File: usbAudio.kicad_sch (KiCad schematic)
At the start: 35 parts, among them J1 USB_B_Micro, J2 54-00176, U1 PCM2906CDBR, U2 MAX9814, U3 TCR2EF36, Y1 12MHz

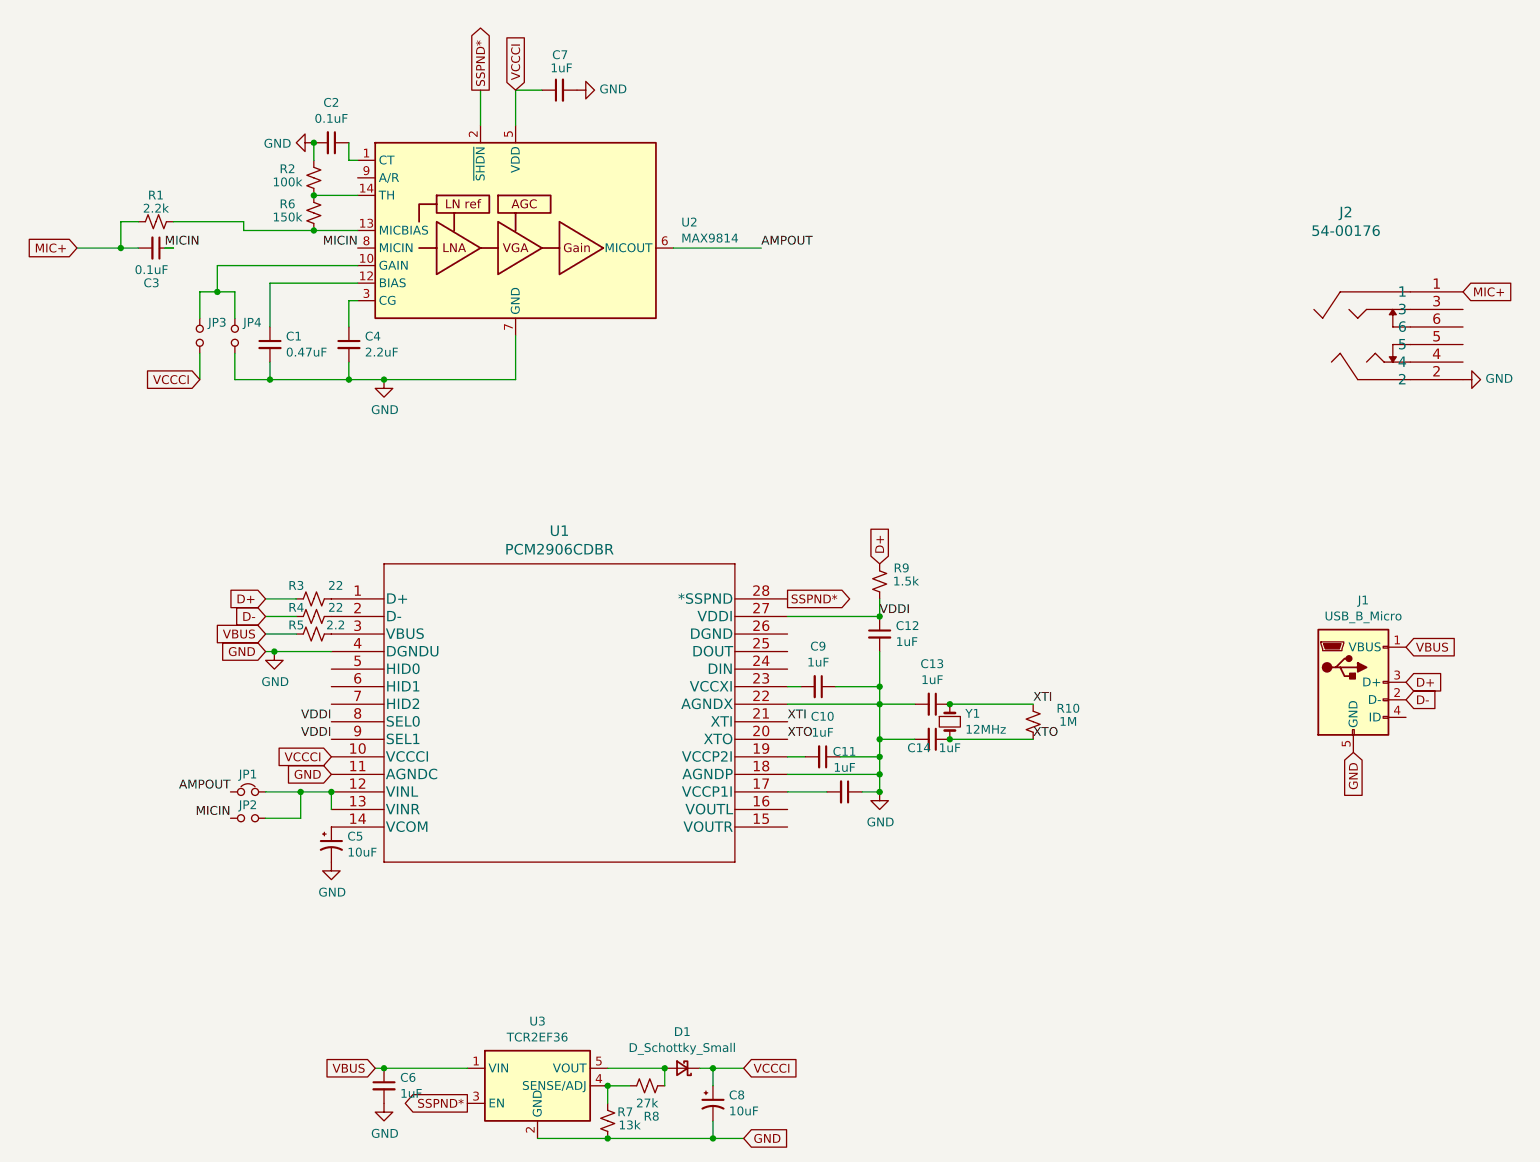
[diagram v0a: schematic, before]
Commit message: Update design and readme
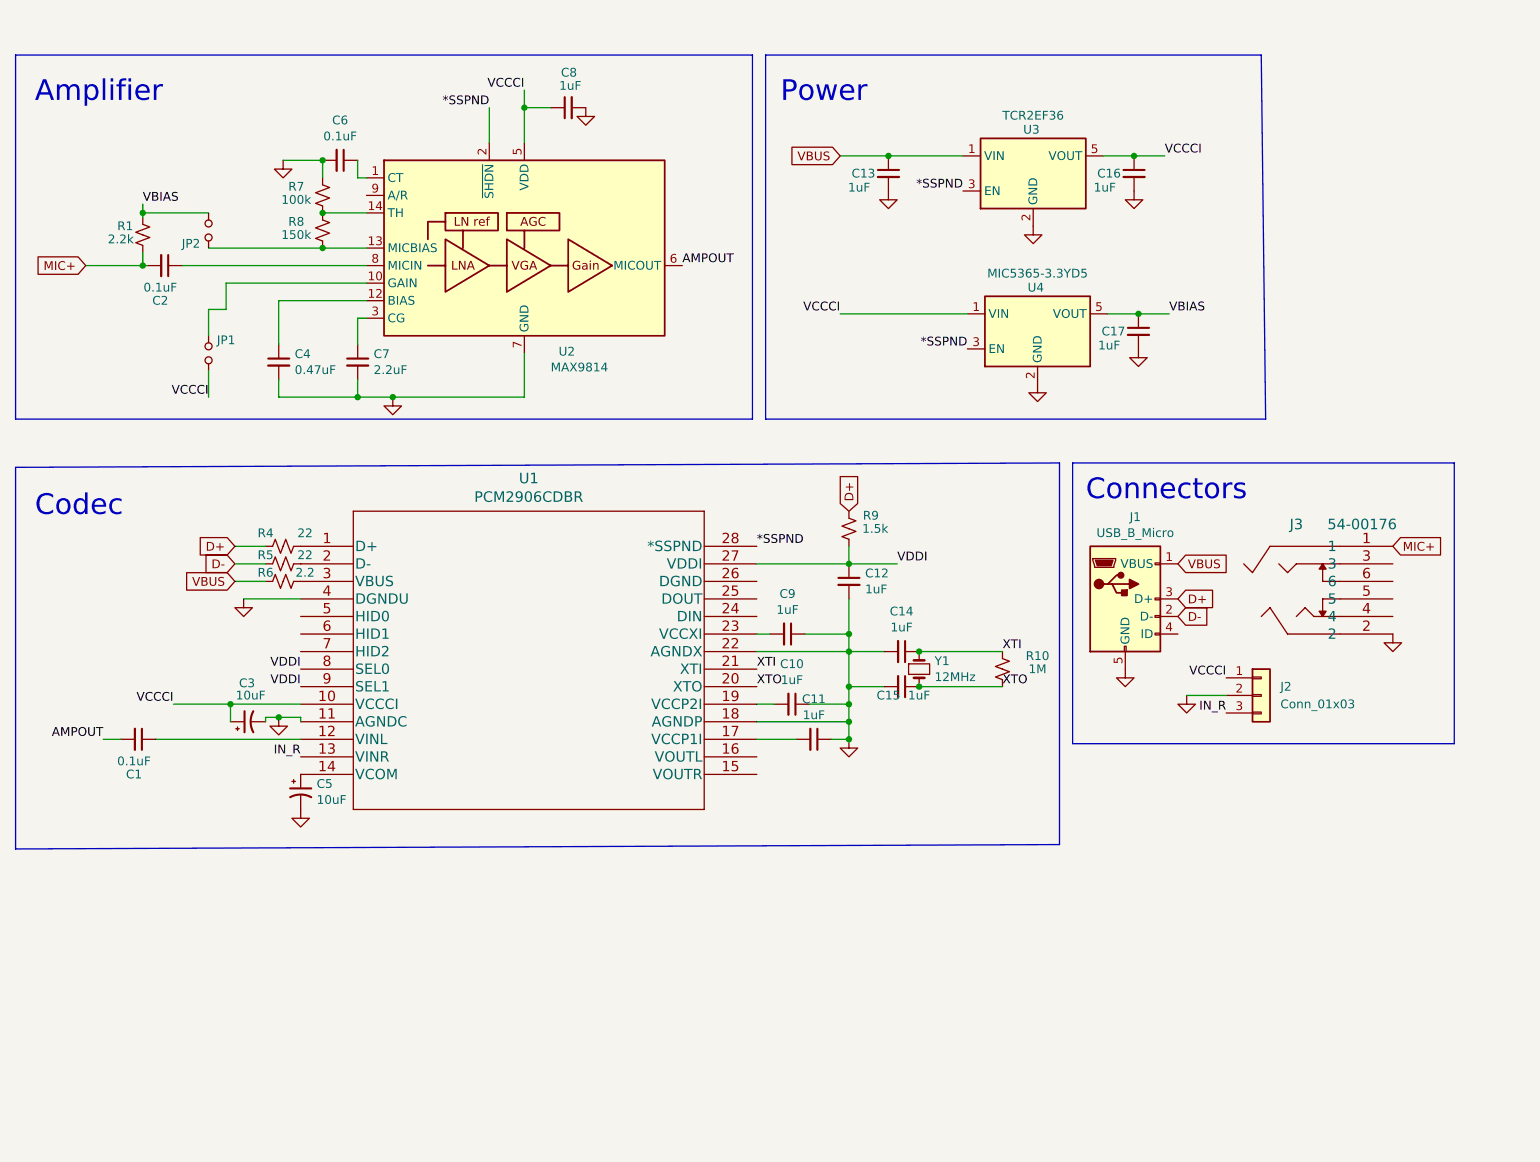
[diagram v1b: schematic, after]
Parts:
- removed C6: 1uF, Capacitor_SMD:C_0603_1608Metric_Pad1.08x0.95mm_HandSolder, symbol Device:C_Small
- removed D1: D_Schottky_Small, Diode_SMD:D_SOD-523, symbol Device:D_Schottky_Small
- removed JP1: Jumper_NC_Small, Jumper:SolderJumper-2_P1.3mm_Bridged_RoundedPad1.0x1.5mm, symbol Device:Jumper_NC_Small
- removed JP4: Jumper_NO_Small, Jumper:SolderJumper-2_P1.3mm_Open_RoundedPad1.0x1.5mm, symbol Device:Jumper_NO_Small
- removed R7: 13k, Resistor_SMD:R_0603_1608Metric_Pad0.98x0.95mm_HandSolder, symbol Device:R_Small_US
- removed R8: 27k, Resistor_SMD:R_0603_1608Metric_Pad0.98x0.95mm_HandSolder, symbol Device:R_Small_US
- removed U3: TCR2EF36, Package_TO_SOT_SMD:TSOT-23-5, symbol Regulator_Linear:ADP7142AUJZ-3.3
- added C1: 0.1uF, Capacitor_SMD:C_0603_1608Metric_Pad1.08x0.95mm_HandSolder, symbol Device:C_Small
- added C13, C16, C17: 1uF, Capacitor_SMD:C_0603_1608Metric_Pad1.08x0.95mm_HandSolder, symbol Device:C_Small
- added J2: Conn_01x03, Package_TO_SOT_THT:TO-92Flat, symbol Connector_Generic:Conn_01x03
- added U3: TCR2EF36, Package_TO_SOT_SMD:SOT-23-5, symbol Regulator_Linear:MIC5365-3.3YD5
- added U4: MIC5365-3.3YD5, Package_TO_SOT_SMD:SOT-23-5, symbol Regulator_Linear:MIC5365-3.3YD5
- renumbered C13 to C14, C14 to C15, C3 to C2, C8 to C3, C1 to C4, C2 to C6, C4 to C7, C7 to C8, J2 to J3, JP3 to JP1, R3 to R4, R4 to R5, R5 to R6, R2 to R7, R6 to R8
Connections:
- net AMPOUT: now also C1.2
- net GND: now also C13.2, C16.2, C17.2, J2.2 (Pin_2), U3.2 (GND), U4.2 (GND)
- net VBUS: now also C13.1, U3.1 (VIN)
- net VCCCI: now also C16.1, J2.1 (Pin_1), U3.5 (VOUT), U4.1 (VIN)
- net at R8.1, U2.13 (MICBIAS): now also JP2.1; no longer R1.1
- net MICIN: no longer names the net of C2.1, U2.8 (MICIN)
- net MICIN: no longer JP2.1
- net SSPND* renamed *SSPND
- net *SSPND: now also U3.3 (EN), U4.3 (EN)
- new net: C1.1, U1.12 (VINL)
- new net IN_R: J2.3 (Pin_3), U1.13 (VINR)
- new net VBIAS: C17.1, JP2.2, R1.1, U4.5 (VOUT)
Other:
- note added: "Amplifier"
- note added: "Codec"
- note added: "Connectors"
- note added: "Power"
- moved on the sheet: C10, C11, C12, C14, C15, C2, C3, C4, C5, C6, C7, C8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
